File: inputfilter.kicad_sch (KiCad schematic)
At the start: 12 parts

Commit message: routed ad2s
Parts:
- R10, R13, R9: LCSC (none) -> C25804
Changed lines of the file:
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@@
+      (effects (font (size 1.27 1.27)) hide)
+    )
+    (property "LCSC" "C25804" (id 4) (at 121.92 83.82 90)
       (effects (font (size 1.27 1.27)) hide)
     )
@@
       (effects (font (size 1.27 1.27)) hide)
     )
+    (property "LCSC" "C25804" (id 4) (at 121.92 121.285 90)
+      (effects (font (size 1.27 1.27)) hide)
+    )
     (pin "1")
     (pin "2")
@@
       (effects (font (size 1.27 1.27)) hide)
     )
+    (property "LCSC" "C25804" (id 4) (at 187.325 96.52 90)
+      (effects (font (size 1.27 1.27)) hide)
+    )

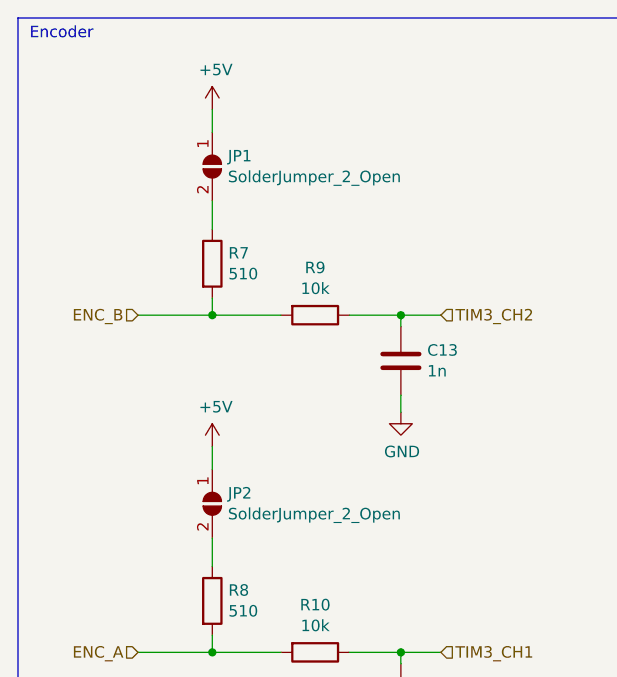
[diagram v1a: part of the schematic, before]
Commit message: fixes for v5
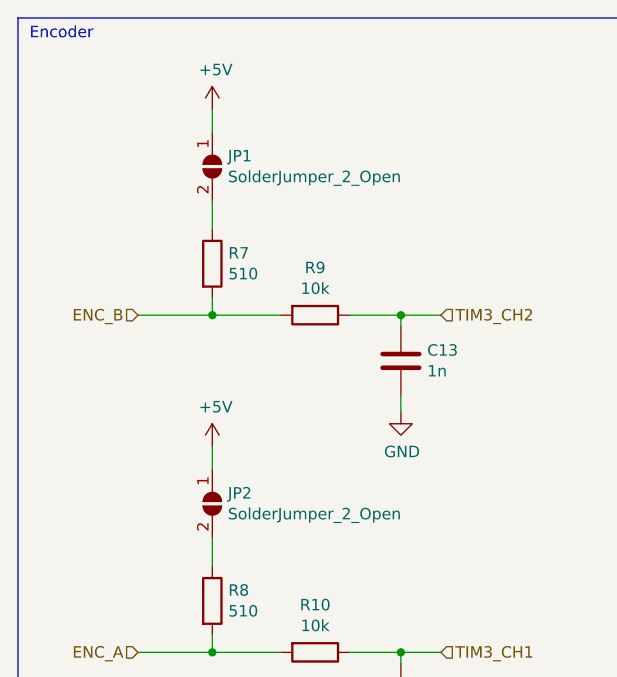
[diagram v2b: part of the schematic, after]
